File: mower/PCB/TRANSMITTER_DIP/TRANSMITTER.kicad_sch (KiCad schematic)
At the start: 14 parts, among them J1 BOT POWER, J2 POWER IN, J3 SHUNT, J4 COIL OUT, J5 COIL POWER IN, Q1 IRF3205, U1 LM358, U4 LM555xN

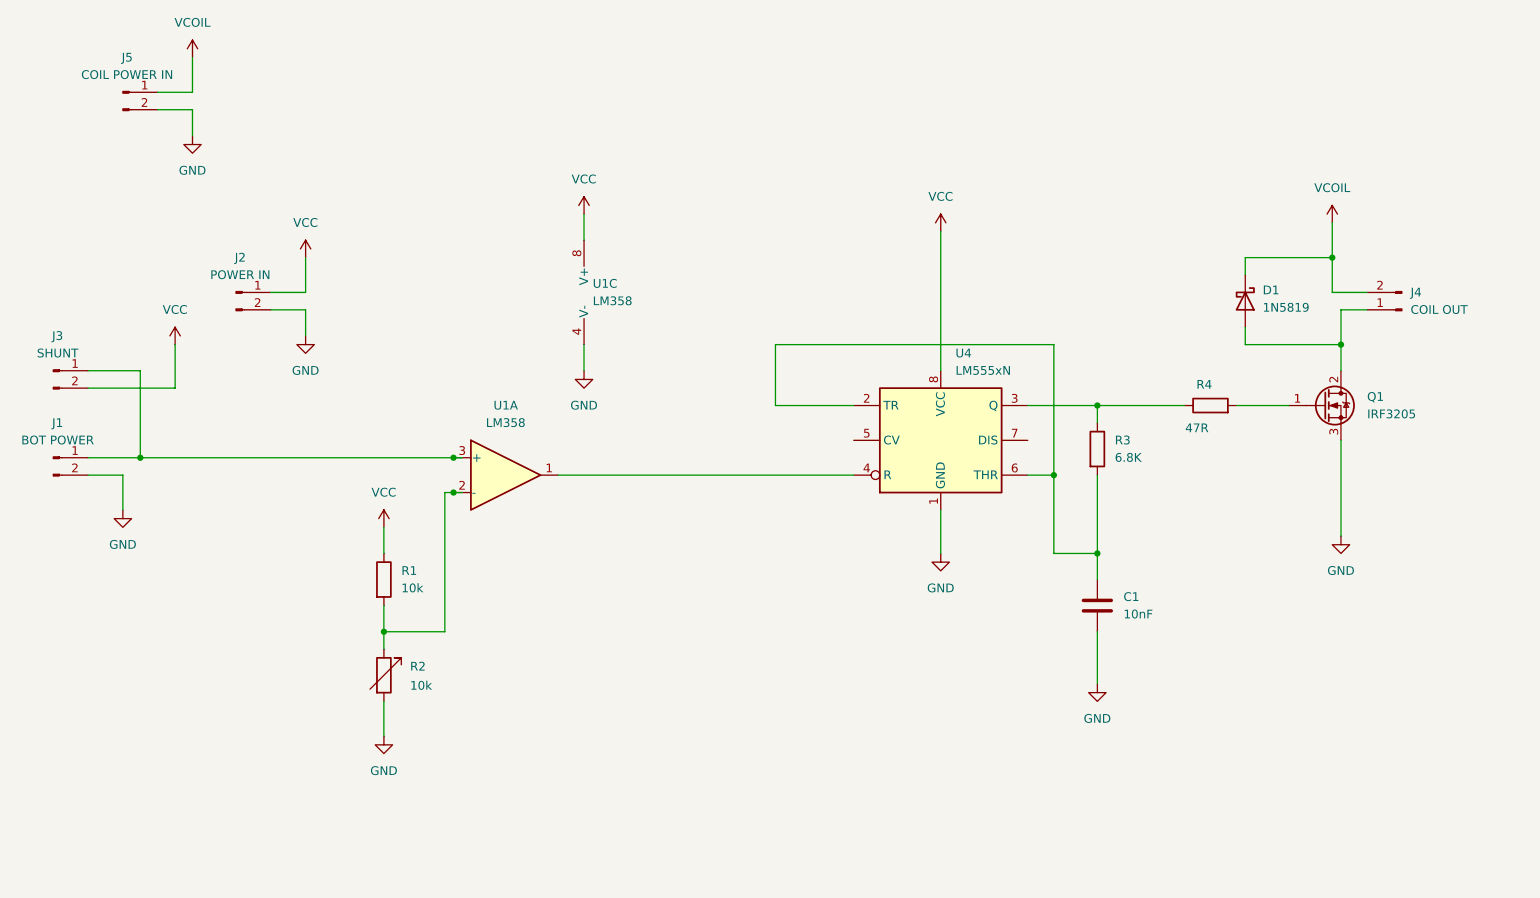
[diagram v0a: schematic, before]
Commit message: .
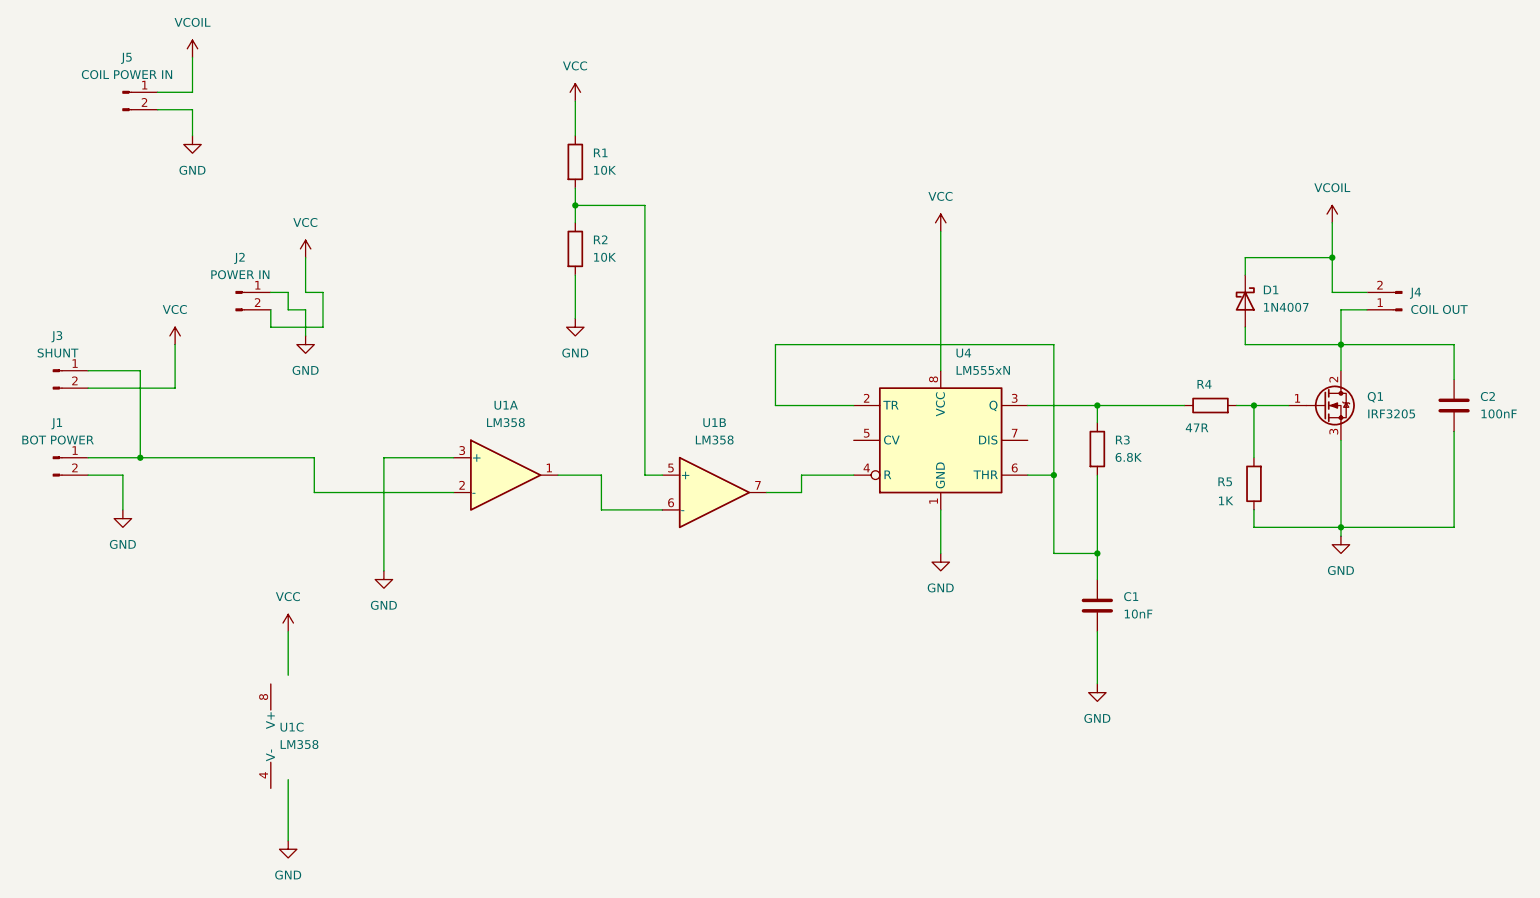
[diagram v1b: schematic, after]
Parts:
- removed R2: 10k, IMRANS_LIBRARY:Potentiometer_Bourns_3386P_Vertical, symbol Device:R_Variable
- added C2: 100nF, IMRANS_LIBRARY:C_Disc_D3.0mm_W1.6mm_P2.50mm, symbol Device:C
- added R2: 10K, IMRANS_LIBRARY:R_Axial_DIN0207_L6.3mm_D2.5mm_P10.16mm_Horizontal_2, symbol Device:R
- added R5: 1K, IMRANS_LIBRARY:R_Axial_DIN0207_L6.3mm_D2.5mm_P10.16mm_Horizontal_2, symbol Device:R
- added unit 2 of U1
- D1: value 1N5819 -> 1N4007
- R1: value 10k -> 10K
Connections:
- net GND: now also J2.1 (Pin_1), U1.3 (+), C2.2, R2.2, R5.1; no longer J2.2 (Pin_2), U1.4 (V-)
- net VCC: now also J2.2 (Pin_2); no longer J2.1 (Pin_1), U1.8 (V+)
- net at U4.4 (R): now also U1.7; no longer U1.1
- net at Q1.1 (G), R4.2: now also R5.2
- net at D1.2 (A), J4.1 (Pin_1), Q1.2 (D): now also C2.1
- net at J1.1 (Pin_1), J3.1 (Pin_1): now also U1.2 (-); no longer U1.3 (+)
- net at R1.2: now also R2.1, U1.5 (+); no longer U1.2 (-)
- new net: U1.1, U1.6 (-)
